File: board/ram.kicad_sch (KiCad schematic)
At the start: 16 parts, among them U10 RAM 4 LO, U11 RAM 4 HI, U4 RAM 1 LO, U5 RAM 1 HI, U6 RAM 2 LO, U7 RAM 2 HI, U8 RAM 3 LO, U9 RAM 3 HI

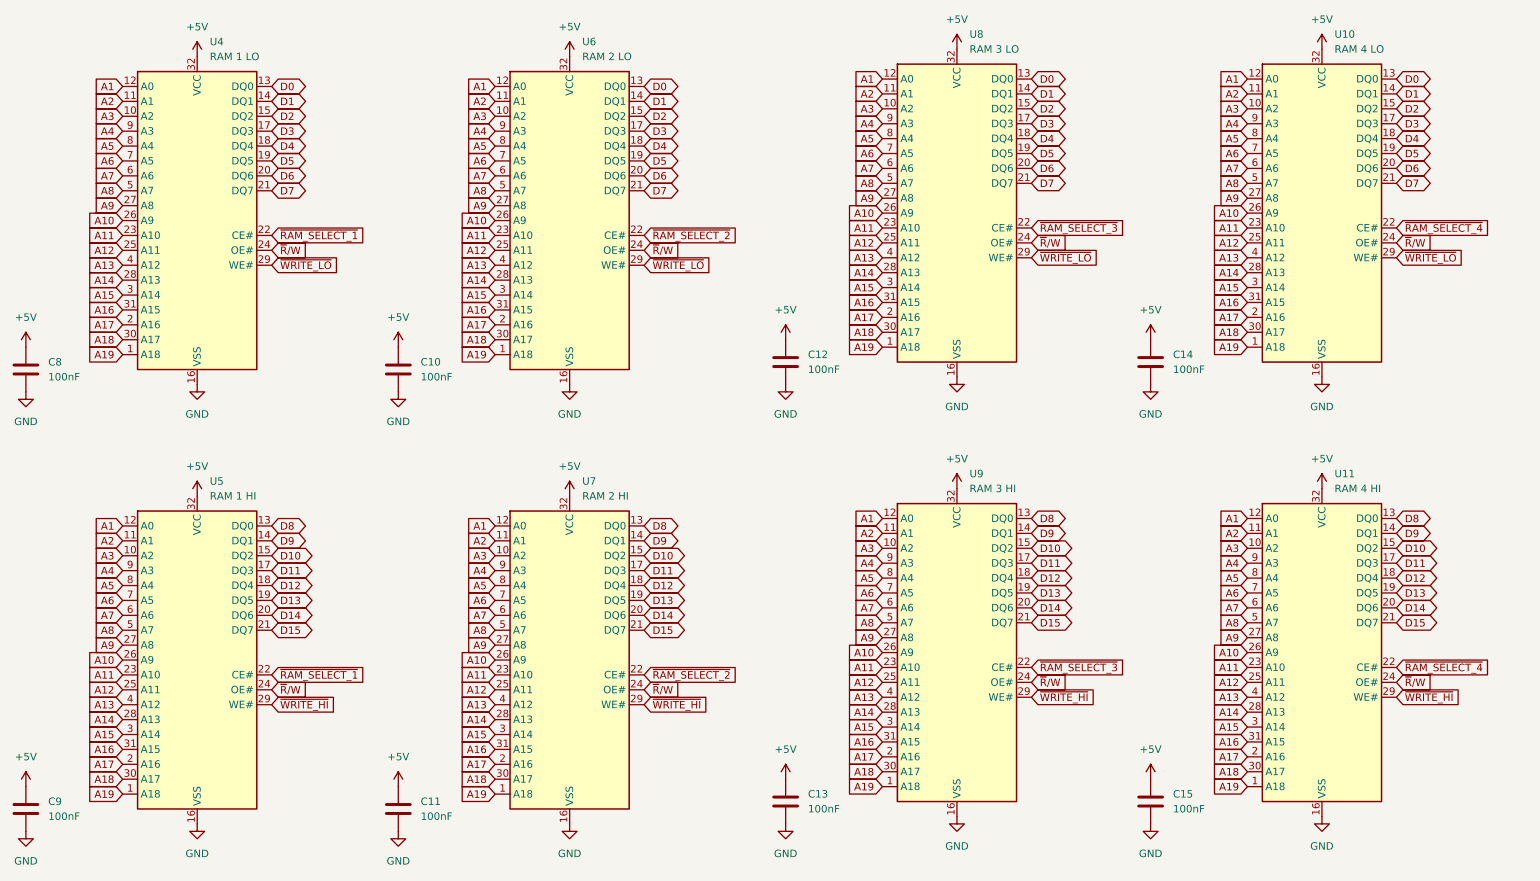
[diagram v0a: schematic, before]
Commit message: checkpoint
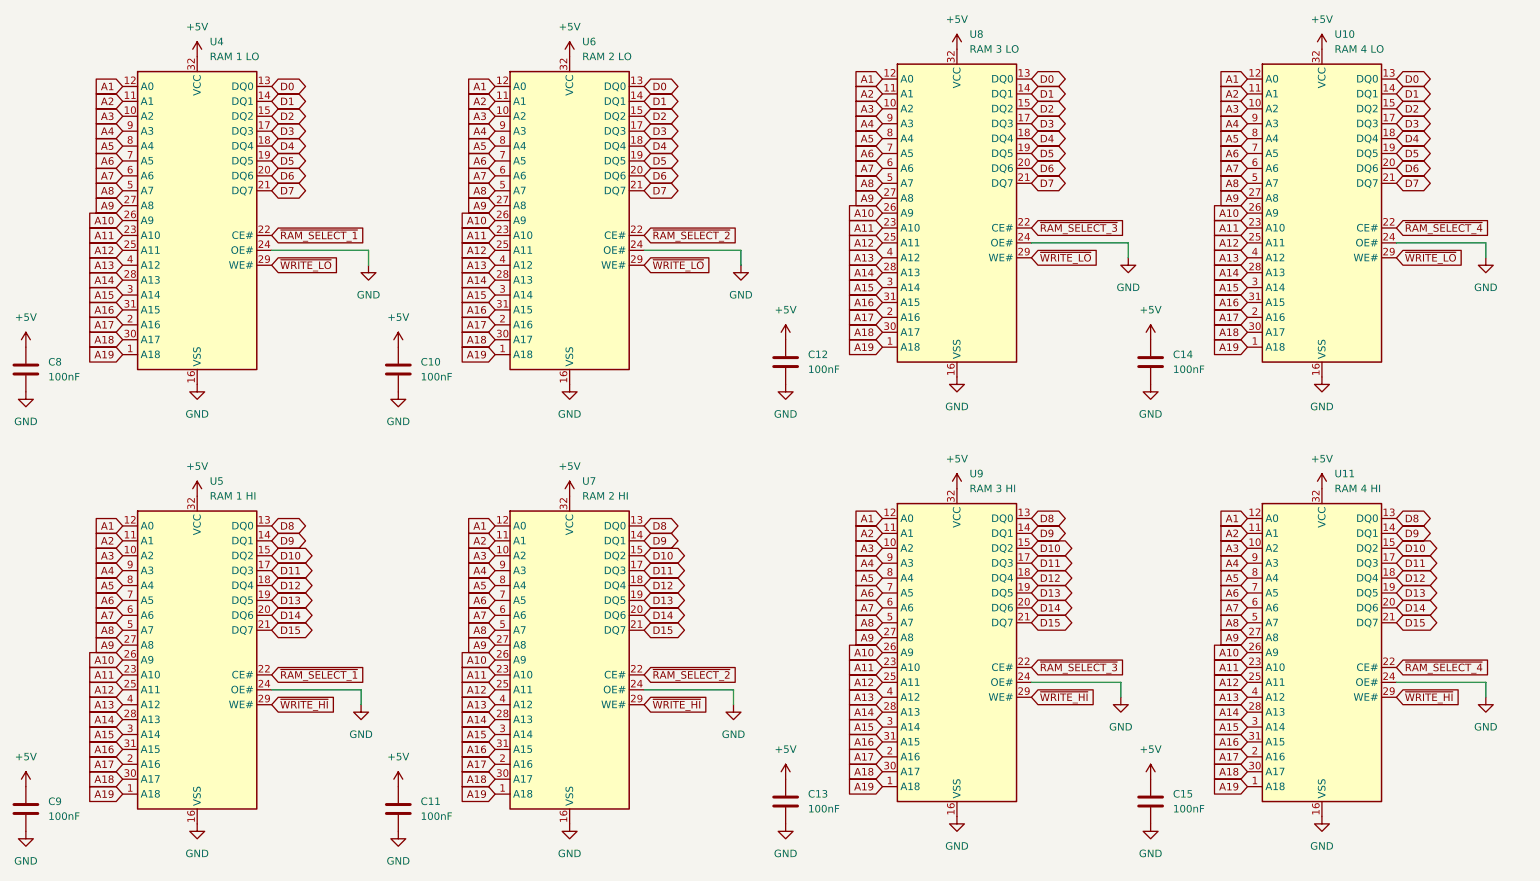
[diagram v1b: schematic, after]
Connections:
- net ~{R}/W is gone; now on net GND: U10.24 (OE#), U11.24 (OE#), U4.24 (OE#), U5.24 (OE#), U6.24 (OE#), U7.24 (OE#), U8.24 (OE#), U9.24 (OE#)
